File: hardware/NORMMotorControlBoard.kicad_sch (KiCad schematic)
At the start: 31 parts, among them J1 Front Right Motor, J2 Front Left Motor, J3 Back Right Motor, J4 Back Left Motor, J5 Conn_01x02_Socket, J6 SparePins, SW1 Reset, U1 Front Driver, U2 Back Driver, U3 74HCT595

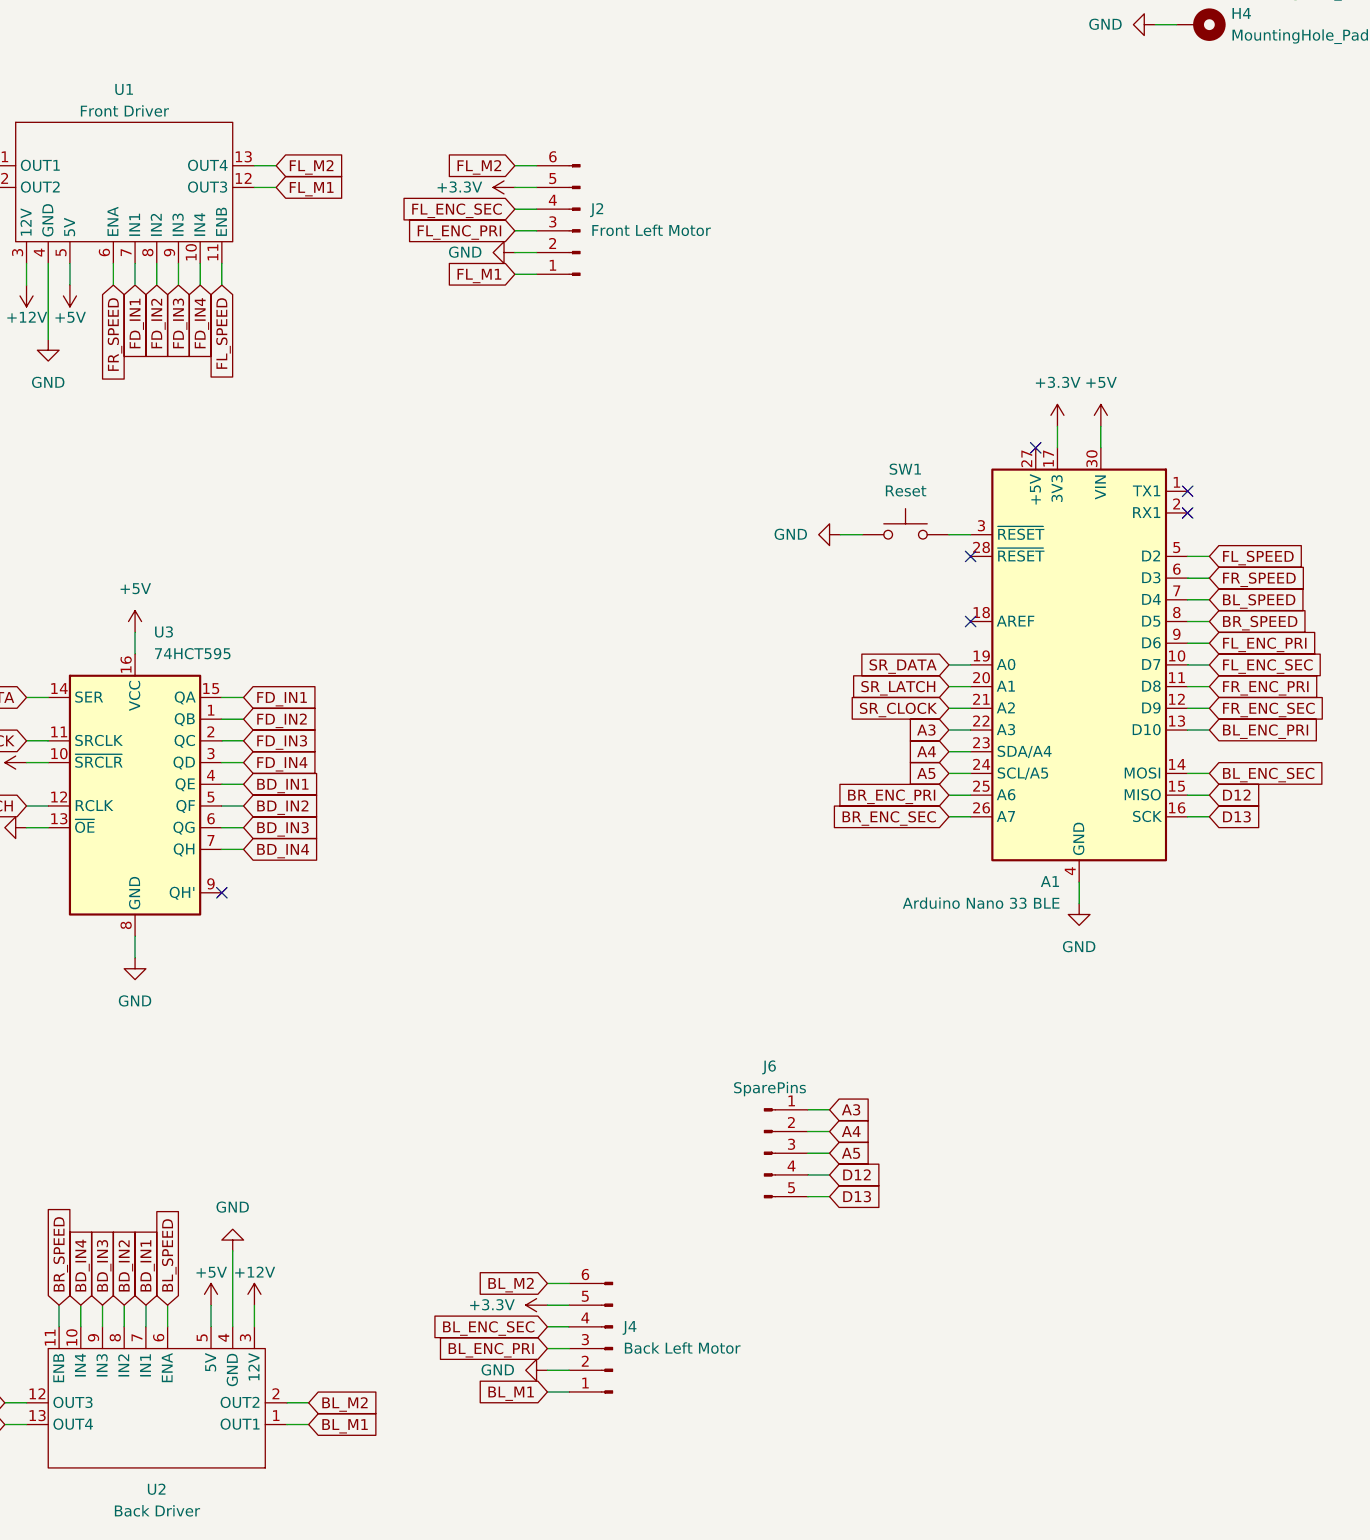
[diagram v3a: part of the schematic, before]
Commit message: Placed components
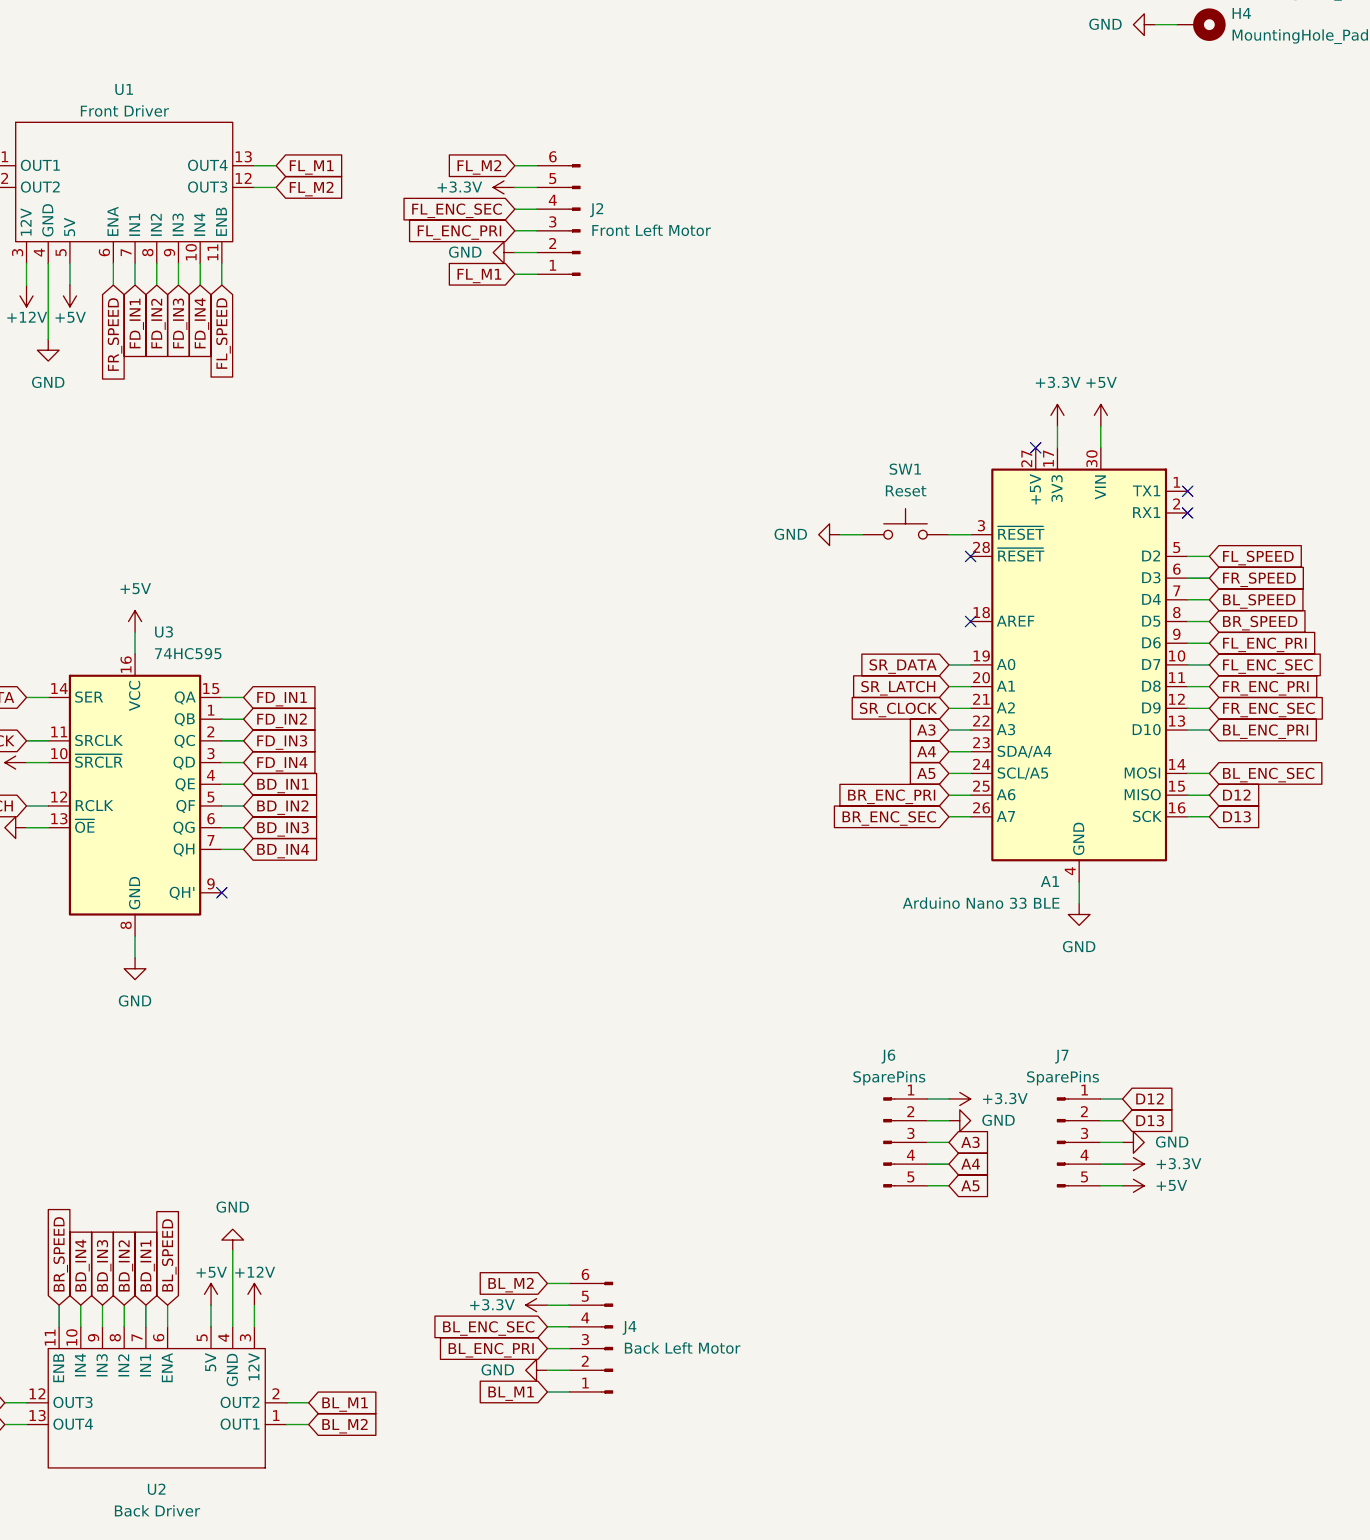
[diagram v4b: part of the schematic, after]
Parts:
- added J7: SparePins, Connector_PinHeader_2.54mm:PinHeader_1x05_P2.54mm_Vertical, symbol Connector:Conn_01x05_Pin
- J6: footprint Connector_PinHeader_2.54mm:PinHeader_1x05_P2.54mm_Vertical -> Connector_PinHeader_2.54mm:PinHeader_1x05_P2.54mm_Horizontal
- U3: value 74HCT595 -> 74HC595; footprint Package_SO:SOIC-16_3.9x9.9mm_P1.27mm -> Package_DIP:DIP-16_W7.62mm; symbol 74xx:74HCT595 -> 74xx:74HC595
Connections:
- net +3.3V: now also J6.1 (Pin_1), J7.4 (Pin_4)
- net +5V: now also J7.5 (Pin_5)
- net A3: now also J6.3 (Pin_3); no longer J6.1 (Pin_1)
- net A4: now also J6.4 (Pin_4); no longer J6.2 (Pin_2)
- net A5: now also J6.5 (Pin_5); no longer J6.3 (Pin_3)
- net BL_M1: now also U2.2 (OUT2); no longer U2.1 (OUT1)
- net BL_M2: now also U2.1 (OUT1); no longer U2.2 (OUT2)
- net D12: now also J7.1 (Pin_1); no longer J6.4 (Pin_4)
- net D13: now also J7.2 (Pin_2); no longer J6.5 (Pin_5)
- net FL_M1: now also U1.13 (OUT4); no longer U1.12 (OUT3)
- net FL_M2: now also U1.12 (OUT3); no longer U1.13 (OUT4)
- net GND: now also J6.2 (Pin_2), J7.3 (Pin_3)
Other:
- moved on the sheet: J6
